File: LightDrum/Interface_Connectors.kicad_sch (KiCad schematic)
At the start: 3 parts, among them J2 0525593652, J3 0541323662, J4 PWR-CONN

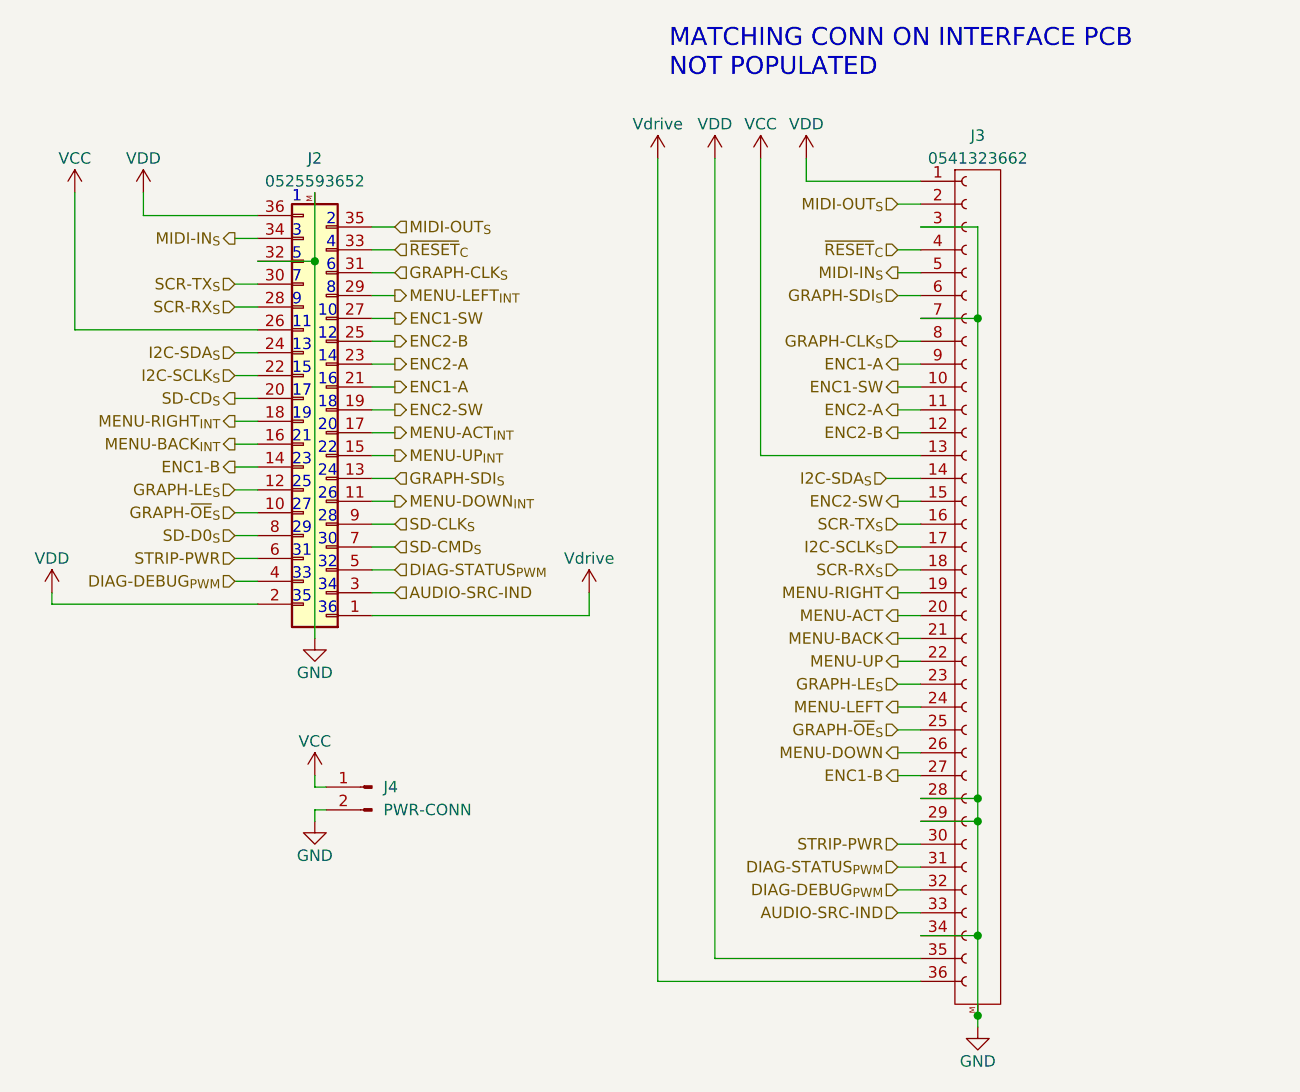
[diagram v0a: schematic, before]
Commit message: PCB Lock REV11
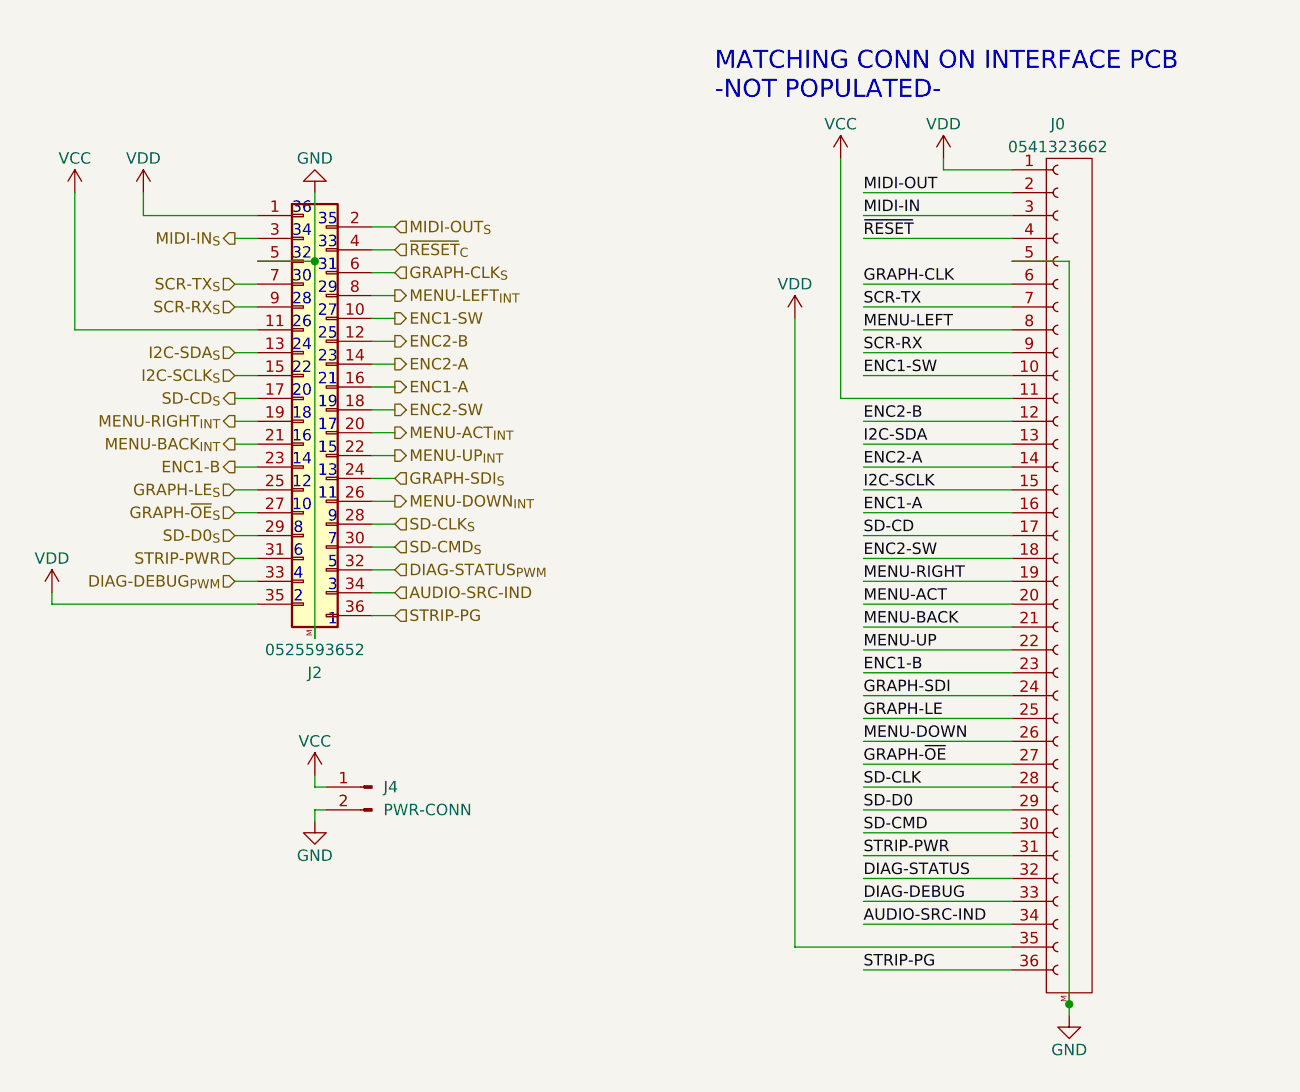
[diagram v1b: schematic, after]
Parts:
- removed J3: 0541323662, Daxxn_Connectors:0541323662, symbol Daxxn_Connectors:0541323662
- added J0: 0541323662, Daxxn_Connectors:0541323662, symbol Daxxn_Connectors:0541323662
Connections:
- net Vdrive is gone; now on net VDD: J2.1 (Pin_1)
- net AUDIO-SRC-IND: now also J2.34 (Pin_34), J0.34 (Pin_34); no longer J2.3 (Pin_3)
- net DIAG-DEBUG_{PWM}: now also J2.33 (Pin_33); no longer J2.4 (Pin_4)
- net DIAG-STATUS_{PWM}: now also J2.32 (Pin_32); no longer J2.5 (Pin_5)
- net ENC1-A: now also J2.16 (Pin_16), J0.16 (Pin_16); no longer J2.21 (Pin_21)
- net ENC1-B: now also J2.23 (Pin_23), J0.23 (Pin_23); no longer J2.14 (Pin_14)
- net ENC1-SW: now also J2.10 (Pin_10), J0.10 (Pin_10); no longer J2.27 (Pin_27)
- net ENC2-A: now also J2.14 (Pin_14), J0.14 (Pin_14); no longer J2.23 (Pin_23)
- net ENC2-B: now also J2.12 (Pin_12), J0.12 (Pin_12); no longer J2.25 (Pin_25)
- net ENC2-SW: now also J2.18 (Pin_18), J0.18 (Pin_18); no longer J2.19 (Pin_19)
- net GND: now also J2.5 (Pin_5), J0.5 (Pin_5), J0.M (MNT); no longer J2.32 (Pin_32)
- net GRAPH-CLK_{S}: now also J2.6 (Pin_6); no longer J2.31 (Pin_31)
- net GRAPH-LE_{S}: now also J2.25 (Pin_25); no longer J2.12 (Pin_12)
- net GRAPH-SDI_{S}: now also J2.24 (Pin_24); no longer J2.13 (Pin_13)
- net GRAPH-~{OE}_{S}: now also J2.27 (Pin_27); no longer J2.10 (Pin_10)
- net I2C-SCLK_{S}: now also J2.15 (Pin_15); no longer J2.22 (Pin_22)
- net I2C-SDA_{S}: now also J2.13 (Pin_13); no longer J2.24 (Pin_24)
- net MENU-ACT: now also J0.20 (Pin_20)
- net MENU-ACT_{INT}: now also J2.20 (Pin_20); no longer J2.17 (Pin_17)
- net MENU-BACK: now also J0.21 (Pin_21)
- net MENU-BACK_{INT}: now also J2.21 (Pin_21); no longer J2.16 (Pin_16)
- net MENU-DOWN: now also J0.26 (Pin_26)
- net MENU-DOWN_{INT}: now also J2.26 (Pin_26); no longer J2.11 (Pin_11)
- net MENU-LEFT: now also J0.8 (Pin_8)
- net MENU-LEFT_{INT}: now also J2.8 (Pin_8); no longer J2.29 (Pin_29)
- net MENU-RIGHT: now also J0.19 (Pin_19)
- net MENU-RIGHT_{INT}: now also J2.19 (Pin_19); no longer J2.18 (Pin_18)
- net MENU-UP: now also J0.22 (Pin_22)
- net MENU-UP_{INT}: now also J2.22 (Pin_22); no longer J2.15 (Pin_15)
- net MIDI-IN_{S}: now also J2.3 (Pin_3); no longer J2.34 (Pin_34)
- net MIDI-OUT_{S}: now also J2.2 (Pin_2); no longer J2.35 (Pin_35)
- net SCR-RX_{S}: now also J2.9 (Pin_9); no longer J2.28 (Pin_28)
- net SCR-TX_{S}: now also J2.7 (Pin_7); no longer J2.30 (Pin_30)
- net SD-CD_{S}: now also J2.17 (Pin_17); no longer J2.20 (Pin_20)
- net SD-CLK_{S}: now also J2.28 (Pin_28); no longer J2.9 (Pin_9)
- net SD-CMD_{S}: now also J2.30 (Pin_30); no longer J2.7 (Pin_7)
- net SD-D0_{S}: now also J2.29 (Pin_29); no longer J2.8 (Pin_8)
- net STRIP-PWR: now also J2.31 (Pin_31), J0.31 (Pin_31); no longer J2.6 (Pin_6)
- net VCC: now also J2.11 (Pin_11), J0.11 (Pin_11); no longer J2.26 (Pin_26)
- net VDD: now also J2.35 (Pin_35), J0.1 (Pin_1), J0.35 (Pin_35); no longer J2.2 (Pin_2), J2.36 (Pin_36)
- net ~{RESET}_{C}: now also J2.4 (Pin_4); no longer J2.33 (Pin_33)
- new net DIAG-DEBUG: J0.33 (Pin_33)
- new net DIAG-STATUS: J0.32 (Pin_32)
- new net GRAPH-CLK: J0.6 (Pin_6)
- new net GRAPH-LE: J0.25 (Pin_25)
- new net GRAPH-SDI: J0.24 (Pin_24)
- new net GRAPH-~{OE}: J0.27 (Pin_27)
- new net I2C-SCLK: J0.15 (Pin_15)
- new net I2C-SDA: J0.13 (Pin_13)
- new net MIDI-IN: J0.3 (Pin_3)
- new net MIDI-OUT: J0.2 (Pin_2)
- new net SCR-RX: J0.9 (Pin_9)
- new net SCR-TX: J0.7 (Pin_7)
- new net SD-CD: J0.17 (Pin_17)
- new net SD-CLK: J0.28 (Pin_28)
- new net SD-CMD: J0.30 (Pin_30)
- new net SD-D0: J0.29 (Pin_29)
- new net STRIP-PG: J0.36 (Pin_36), J2.36 (Pin_36)
- new net ~{RESET}: J0.4 (Pin_4)
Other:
- note added: "MATCHING CONN ON INTERFACE PCB -NOT POPULATED-"
- note removed: "MATCHING CONN ON INTERFACE PCB NOT POPULATED"
- moved on the sheet: J2
